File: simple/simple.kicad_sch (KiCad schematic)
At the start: 3 parts, among them p1 ${SIM.PARAMS}

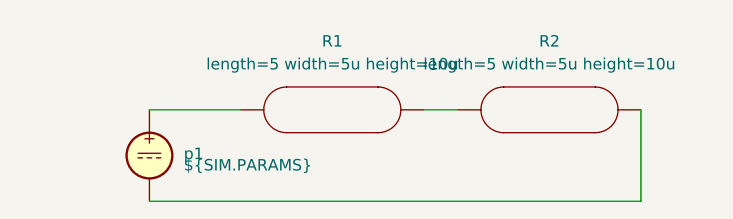
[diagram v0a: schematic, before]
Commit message: WIP
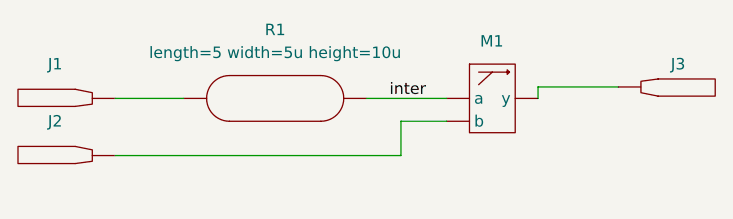
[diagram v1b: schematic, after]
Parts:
- removed R2: ${SIM.PARAMS}, symbol mfda:chamber
- removed p1: ${SIM.PARAMS}, symbol mfda_spice:pressure_source
- added J1, J2, J3: ~, h.r.3.3:pinhole_325px_0, symbol mfda:tube_connector
- added M1: ~, h.r.3.3:diffmix_25px_0, symbol mfda:mixer_2
- R1: footprint (none) -> h.r.3.3:serpentine_50px_0
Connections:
- net at R1.1 (in): now also J1.1 (connect)
- net inter: now reaches R1.2 (out)
- net inter: now also M1.1 (a)
- new net: J3.1 (connect), M1.3 (y)
- new net: J2.1 (connect), M1.2 (b)
